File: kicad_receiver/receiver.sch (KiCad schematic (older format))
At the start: 28 parts, among them J1 Conn_01x05_Male, J2 Conn_01x01, U1 LP2985-3.3, U2 LP2985-3.3, U3 STM32F030F4Px, U4 NRF24L01_Breakout, U5 TP4056, U6 L9110, U7 MT3608

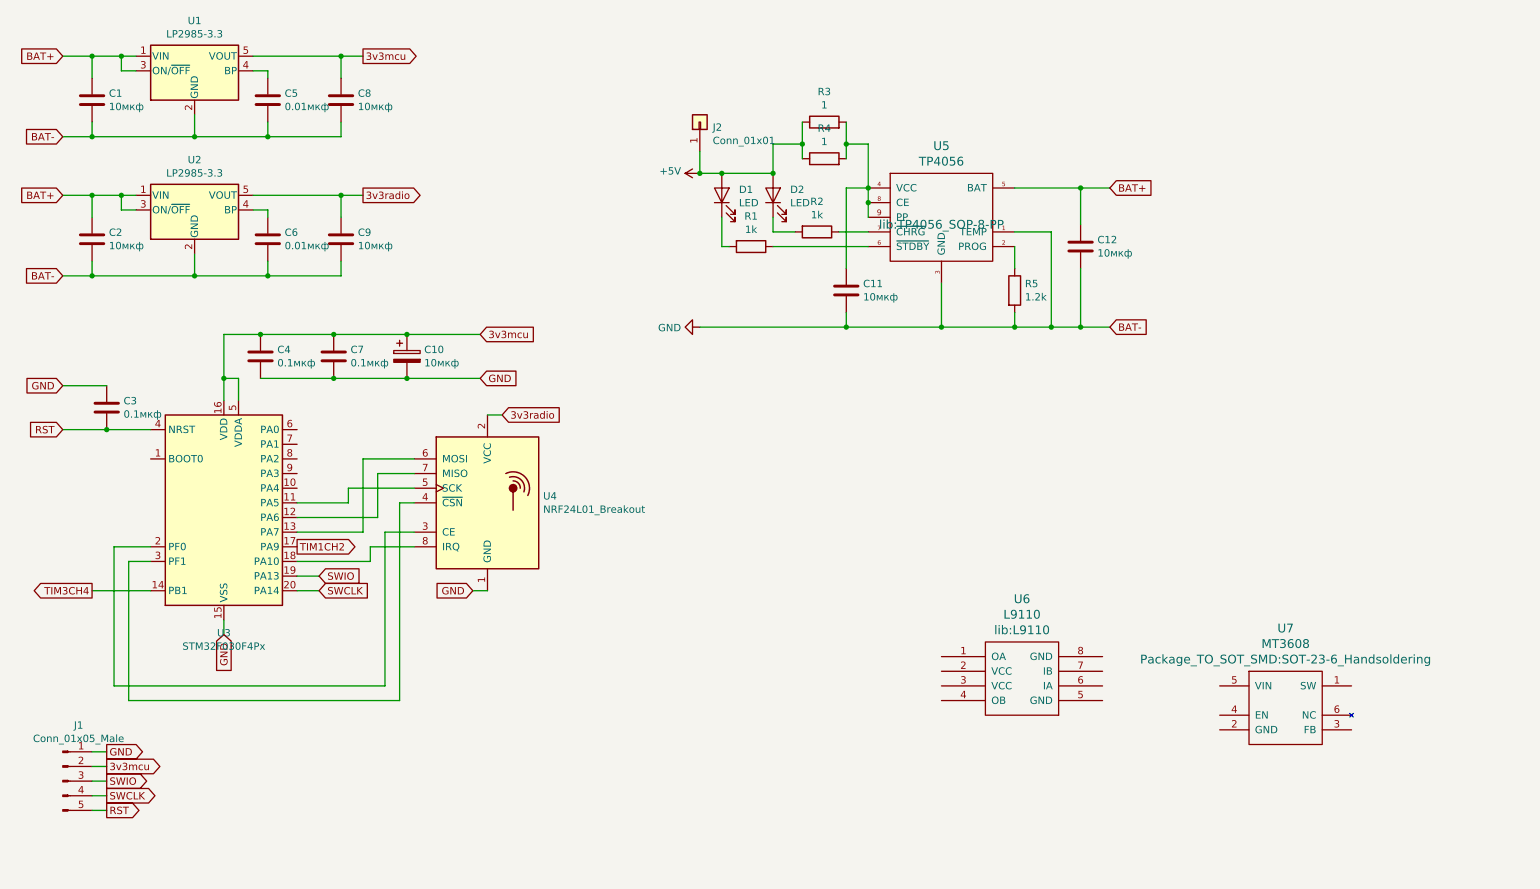
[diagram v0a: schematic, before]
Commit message: more stuff added
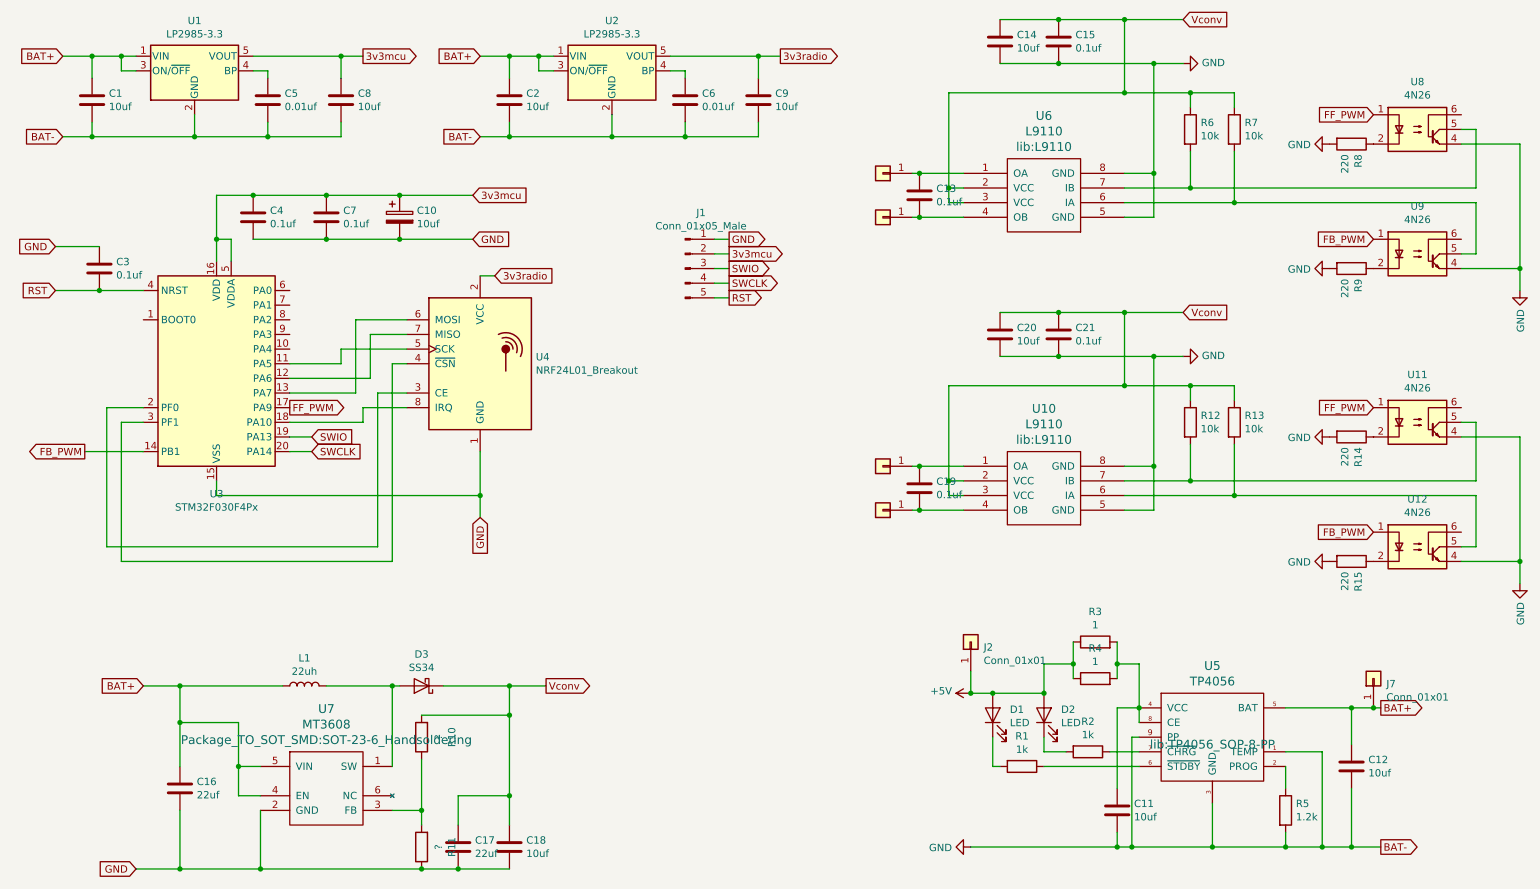
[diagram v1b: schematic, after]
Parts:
- added C13, C15, C19, C21: 0.1uf, Capacitor_SMD:C_0603_1608Metric_Pad1.05x0.95mm_HandSolder, symbol Device:C
- added C14, C20: 10uf, Capacitor_SMD:C_0603_1608Metric_Pad1.05x0.95mm_HandSolder, symbol Device:C
- added C16, C17: 22uf, Capacitor_SMD:C_0805_2012Metric_Pad1.15x1.40mm_HandSolder, symbol Device:C
- added C18: 10uf, Capacitor_SMD:C_0805_2012Metric_Pad1.15x1.40mm_HandSolder, symbol Device:C
- added D3: SS34, Diode_SMD:D_2114_3652Metric, symbol Device:D_Schottky
- added J3, J4, J5, J6, J7: Conn_01x01, Connector_Wire:SolderWirePad_1x01_SMD_5x10mm, symbol Connector_Generic:Conn_01x01
- added L1: 22uh, Inductor_SMD:L_10.4x10.4_H4.8, symbol Device:L
- added R10, R11: ?, Resistor_SMD:R_0603_1608Metric_Pad1.05x0.95mm_HandSolder, symbol Device:R
- added R12, R13, R6, R7: 10k, Resistor_SMD:R_0603_1608Metric_Pad1.05x0.95mm_HandSolder, symbol Device:R
- added R14, R15, R8, R9: 220, Resistor_SMD:R_0603_1608Metric_Pad1.05x0.95mm_HandSolder, symbol Device:R
- added U10: L9110, lib:L9110, symbol L9110:L9110
- added U11, U12, U8, U9: 4N26, Package_DIP:DIP-6_W7.62mm_SMDSocket_SmallPads, symbol Isolator:4N26
- C1, C10, C11, C12, C2, C8, C9: value 10мкф -> 10uf
- C3, C4, C7: value 0.1мкф -> 0.1uf
- C5, C6: value 0.01мкф -> 0.01uf
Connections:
- net BAT+: now also U7.4 (EN), U7.5 (VIN), C16.1, J7.1 (Pin_1), L1.1
- net GND: now also U5.9 (PP), U6.5 (GND), U6.8 (GND), U7.2 (GND), C14.2, C15.2, C16.2, C17.2, C18.2, C20.2, C21.2, R11.1, R14.2, R15.2, R8.2, R9.2, U10.5 (GND), U10.8 (GND), U11.4, U12.4, U8.4, U9.4
- net at C11.1, R3.2, R4.2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: no longer U5.9 (PP)
- net at U6.1 (OA): now also C13.1, J3.1 (Pin_1)
- net Vconv: now reaches U6.2 (VCC)
- net Vconv: now also U6.3 (VCC), C14.1, C15.1, C17.1, C18.1, C20.1, C21.1, D3.1 (K), R10.2, R12.1, R13.1, R6.1, R7.1, U10.2 (VCC), U10.3 (VCC)
- net at U6.4 (OB): now also C13.2, J4.1 (Pin_1)
- net at U6.6 (IA): now also R7.2, U9.5
- net at U6.7 (IB): now also R6.2, U8.5
- net at U7.1 (SW): now also D3.2 (A), L1.2
- net at U7.3 (FB): now also R10.1, R11.2
- net TIM1CH2 renamed FF_PWM
- net FF_PWM: now also U11.1, U8.1
- net TIM3CH4 renamed FB_PWM
- net FB_PWM: now also U12.1, U9.1
- new net: C19.1, J5.1 (Pin_1), U10.1 (OA)
- new net: C19.2, J6.1 (Pin_1), U10.4 (OB)
- new net: R13.2, U10.6 (IA), U12.5
- new net: R12.2, U10.7 (IB), U11.5
- new net: R14.1, U11.2
- new net: R15.1, U12.2
- new net: R8.1, U8.2
- new net: R9.1, U9.2
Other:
- moved on the sheet: C10, C11, C12, C2, C3, C4, C6, C7, C9, D1, D2, J1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
